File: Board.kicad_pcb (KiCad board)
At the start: 2 copper layers, 101.6 x 53.3 mm, 5 parts, among them P1 Relay 1, P2 Relay 2, P3 Relay 3, P4 Relay 4

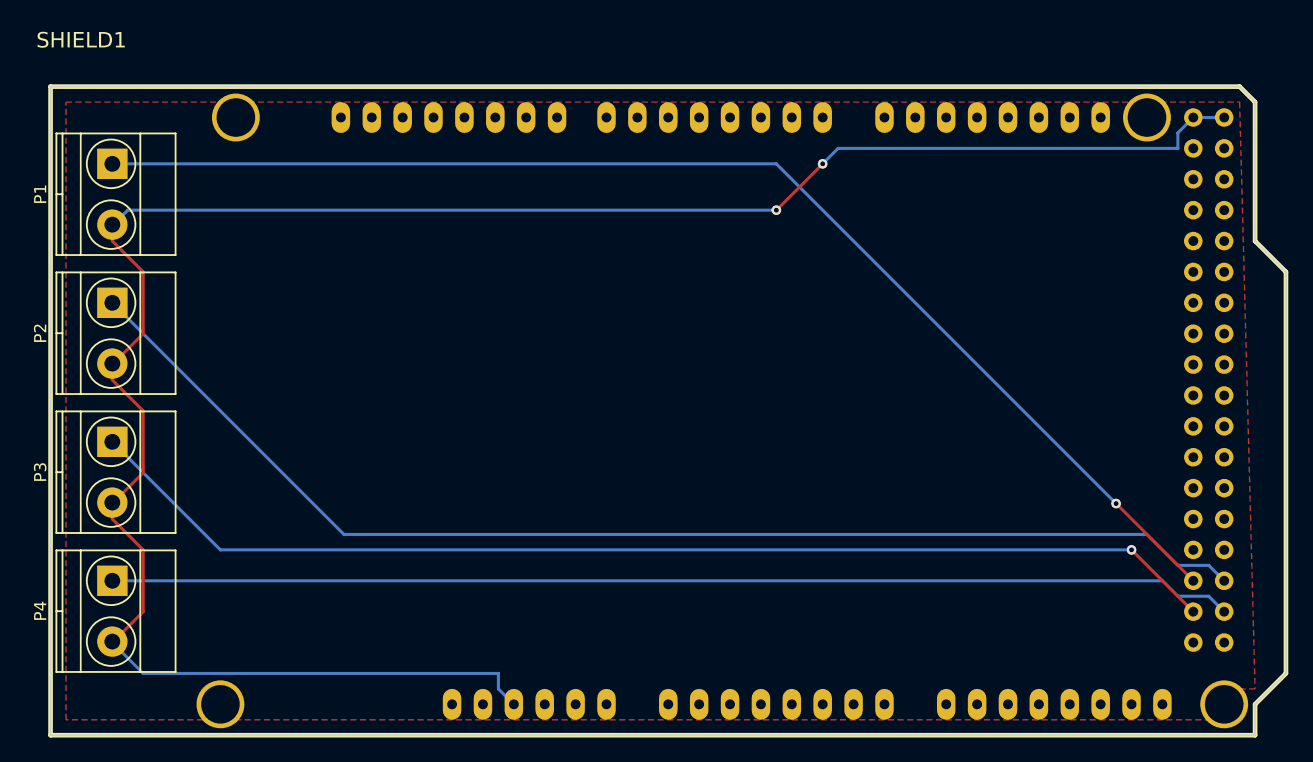
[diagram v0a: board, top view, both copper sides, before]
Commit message: Pins are in
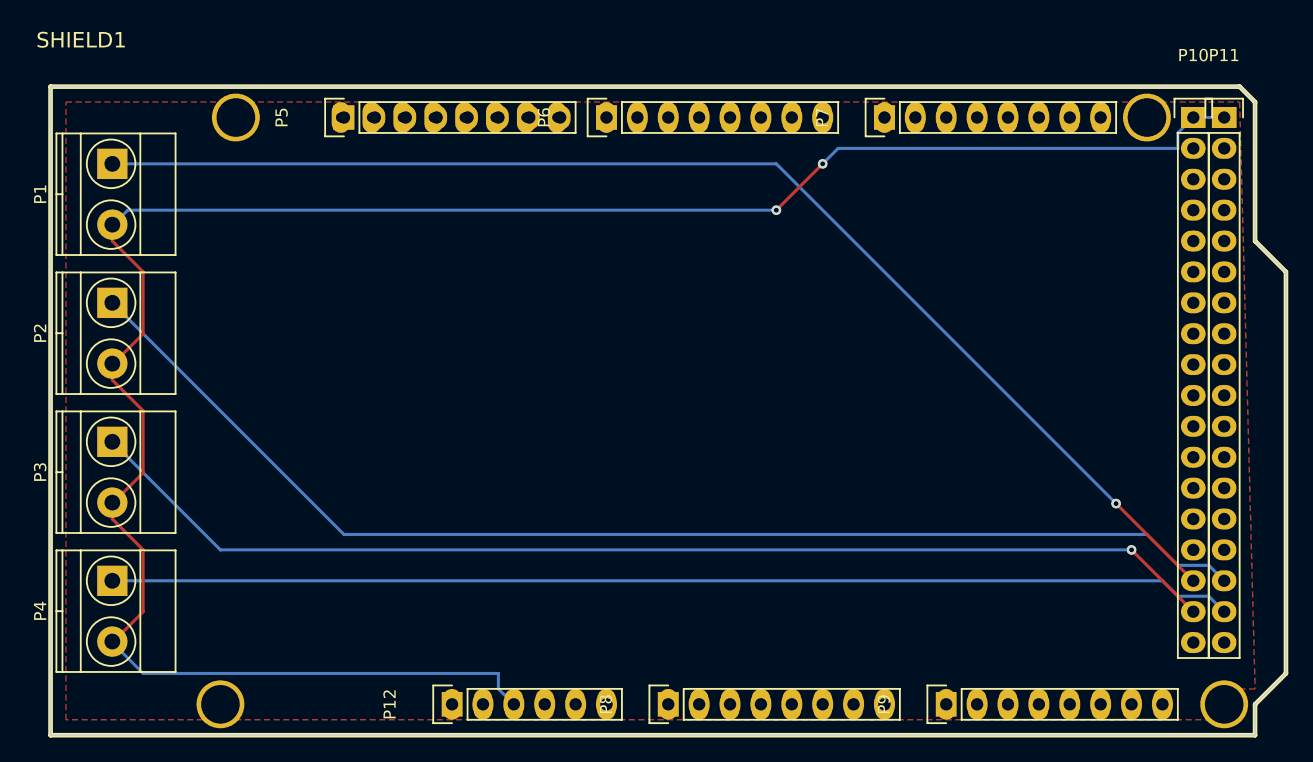
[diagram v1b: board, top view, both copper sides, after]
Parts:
- added P10: CONN_01X18, Pin_Headers:Pin_Header_Straight_1x18, F.Cu at (208.3, 88.9)
- added P11: CONN_01X18, Pin_Headers:Pin_Header_Straight_1x18, F.Cu at (210.8, 88.9)
- added P12: CONN_01X06, Pin_Headers:Pin_Header_Straight_1x06, F.Cu at (147.3, 137.2)
- added P5: CONN_01X08, Pin_Headers:Pin_Header_Straight_1x08, F.Cu at (138.4, 88.9)
- added P6: CONN_01X08, Pin_Headers:Pin_Header_Straight_1x08, F.Cu at (160.0, 88.9)
- added P7: CONN_01X08, Pin_Headers:Pin_Header_Straight_1x08, F.Cu at (182.9, 88.9)
- added P8: CONN_01X08, Pin_Headers:Pin_Header_Straight_1x08, F.Cu at (165.1, 137.2)
- added P9: CONN_01X08, Pin_Headers:Pin_Header_Straight_1x08, F.Cu at (188.0, 137.2)
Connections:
- SHIELD1 pad 0: Net-(SHIELD1-Pad0) -> RX
- SHIELD1 pad 1: Net-(SHIELD1-Pad1) -> TX
- SHIELD1 pad 10: Net-(SHIELD1-Pad10) -> 10
- SHIELD1 pad 11: Net-(SHIELD1-Pad11) -> 11
- SHIELD1 pad 12: Net-(SHIELD1-Pad12) -> 12
- SHIELD1 pad 13: Net-(SHIELD1-Pad13) -> 13
- SHIELD1 pad 14: Net-(SHIELD1-Pad14) -> TX3
- SHIELD1 pad 15: Net-(SHIELD1-Pad15) -> RX3
- SHIELD1 pad 16: Net-(SHIELD1-Pad16) -> TX2
- SHIELD1 pad 17: Net-(SHIELD1-Pad17) -> RX2
- SHIELD1 pad 18: Net-(SHIELD1-Pad18) -> TX1
- SHIELD1 pad 19: Net-(SHIELD1-Pad19) -> RX1
- SHIELD1 pad 2: Net-(SHIELD1-Pad2) -> 2
- SHIELD1 pad 20: Net-(SHIELD1-Pad20) -> SDA
- SHIELD1 pad 21: Net-(SHIELD1-Pad21) -> SCL
- SHIELD1 pad 22: Net-(SHIELD1-Pad22) -> PA0
- SHIELD1 pad 23: Net-(SHIELD1-Pad23) -> PA1
- SHIELD1 pad 24: Net-(SHIELD1-Pad24) -> PA2
- SHIELD1 pad 25: Net-(SHIELD1-Pad25) -> PA3
- SHIELD1 pad 26: Net-(SHIELD1-Pad26) -> PA4
- SHIELD1 pad 27: Net-(SHIELD1-Pad27) -> PA5
- SHIELD1 pad 28: Net-(SHIELD1-Pad28) -> PA6
- SHIELD1 pad 29: Net-(SHIELD1-Pad29) -> PA7
- SHIELD1 pad 3: Net-(SHIELD1-Pad3) -> 3
- SHIELD1 pad 30: Net-(SHIELD1-Pad30) -> PC7
- SHIELD1 pad 31: Net-(SHIELD1-Pad31) -> PC6
- SHIELD1 pad 32: Net-(SHIELD1-Pad32) -> PC5
- SHIELD1 pad 33: Net-(SHIELD1-Pad33) -> PC4
- SHIELD1 pad 34: Net-(SHIELD1-Pad34) -> PC3
- SHIELD1 pad 35: Net-(SHIELD1-Pad35) -> PC2
- SHIELD1 pad 36: Net-(SHIELD1-Pad36) -> PC1
- SHIELD1 pad 37: Net-(SHIELD1-Pad37) -> PC0
- SHIELD1 pad 38: Net-(SHIELD1-Pad38) -> PD7
- SHIELD1 pad 39: Net-(SHIELD1-Pad39) -> PG2
- SHIELD1 pad 3V3: Net-(SHIELD1-Pad3V3) -> 3V
- SHIELD1 pad 4: Net-(SHIELD1-Pad4) -> 4
- SHIELD1 pad 40: Net-(SHIELD1-Pad40) -> PG1
- SHIELD1 pad 41: Net-(SHIELD1-Pad41) -> PG0
- SHIELD1 pad 42: Net-(SHIELD1-Pad42) -> PL7
- SHIELD1 pad 43: Net-(SHIELD1-Pad43) -> PL6
- SHIELD1 pad 44: Net-(SHIELD1-Pad44) -> PL5
- SHIELD1 pad 45: Net-(SHIELD1-Pad45) -> PL4
- SHIELD1 pad 46: Net-(SHIELD1-Pad46) -> PL3
- SHIELD1 pad 47: Net-(SHIELD1-Pad47) -> PL2
- SHIELD1 pad 48: Net-(SHIELD1-Pad48) -> PL1
- SHIELD1 pad 49: Net-(SHIELD1-Pad49) -> PL0
- SHIELD1 pad 5: Net-(SHIELD1-Pad5) -> 5
- SHIELD1 pad 6: Net-(SHIELD1-Pad6) -> 6
- SHIELD1 pad 7: Net-(SHIELD1-Pad7) -> 7
- SHIELD1 pad 8: Net-(SHIELD1-Pad8) -> 8
- SHIELD1 pad 9: Net-(SHIELD1-Pad9) -> 9
- SHIELD1 pad AD0: Net-(SHIELD1-PadAD0) -> AD0
- SHIELD1 pad AD1: Net-(SHIELD1-PadAD1) -> AD1
- SHIELD1 pad AD10: Net-(SHIELD1-PadAD10) -> AD10
- SHIELD1 pad AD11: Net-(SHIELD1-PadAD11) -> AD11
- SHIELD1 pad AD12: Net-(SHIELD1-PadAD12) -> AD12
- SHIELD1 pad AD13: Net-(SHIELD1-PadAD13) -> AD13
- SHIELD1 pad AD14: Net-(SHIELD1-PadAD14) -> AD14
- SHIELD1 pad AD15: Net-(SHIELD1-PadAD15) -> AD15
- SHIELD1 pad AD2: Net-(SHIELD1-PadAD2) -> AD2
- SHIELD1 pad AD3: Net-(SHIELD1-PadAD3) -> AD3
- SHIELD1 pad AD4: Net-(SHIELD1-PadAD4) -> AD4
- SHIELD1 pad AD5: Net-(SHIELD1-PadAD5) -> AD5
- SHIELD1 pad AD6: Net-(SHIELD1-PadAD6) -> AD6
- SHIELD1 pad AD7: Net-(SHIELD1-PadAD7) -> AD7
- SHIELD1 pad AD8: Net-(SHIELD1-PadAD8) -> AD8
- SHIELD1 pad AD9: Net-(SHIELD1-PadAD9) -> AD9
- SHIELD1 pad AREF: Net-(SHIELD1-PadAREF) -> AREF
- SHIELD1 pad RST: Net-(SHIELD1-PadRST) -> RST
- SHIELD1 pad V_IN: Net-(SHIELD1-PadV_IN) -> V_IN
